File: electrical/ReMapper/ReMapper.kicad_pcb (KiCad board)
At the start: 4 copper layers, 35 x 65 mm, 43 parts, among them J1 ESP_UART0, J2 I2C Display, J3 USB_IN, J4 USB_OUT, J5 Button GND Pad, J9 Button Socket, U1 SPX1117M3-L-3-3/TR, U2 W25Q128JVE, U3 ESP32-S3-WROOM-1-N8R8, U4 RP2040, U5 W25Q128JVE, Y1 12MHZ

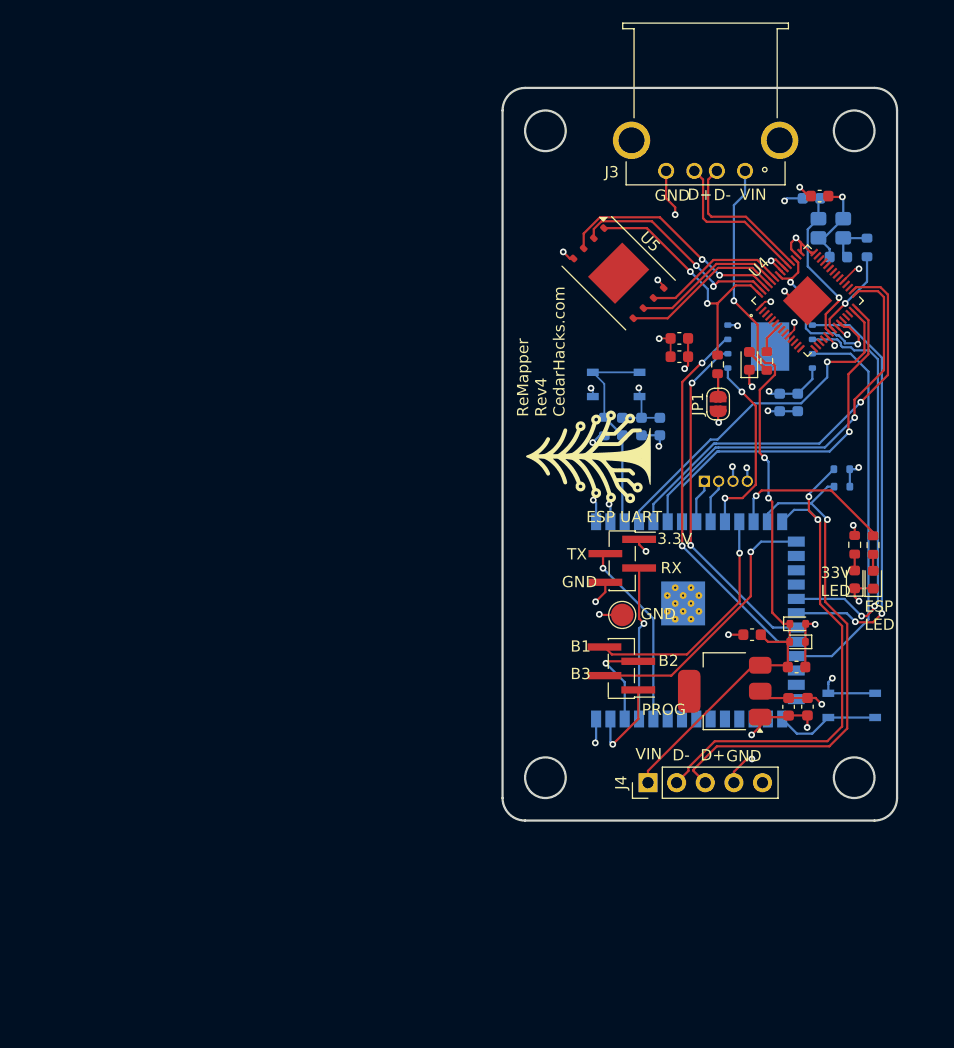
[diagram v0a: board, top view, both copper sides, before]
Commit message: started working on v5
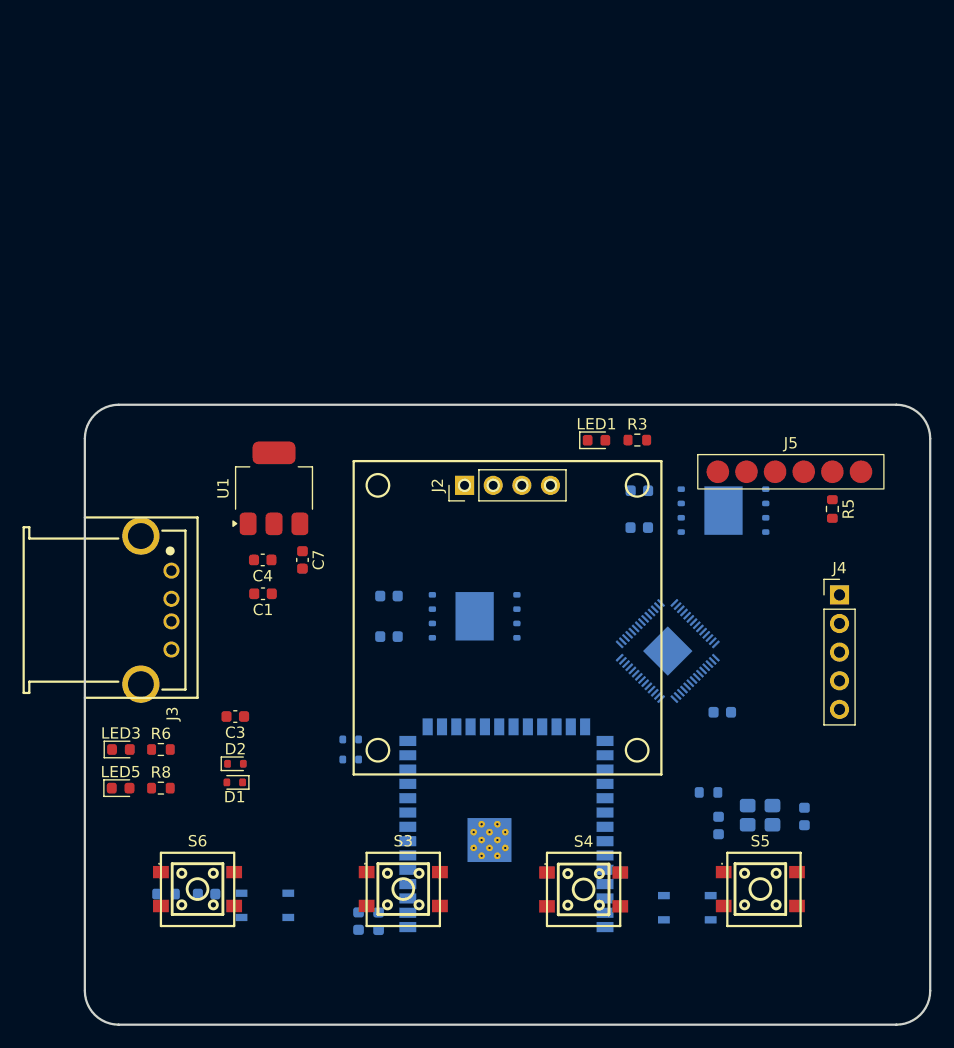
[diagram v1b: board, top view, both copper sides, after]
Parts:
- removed G***: LOGO, LOGO
- removed J1: ESP_UART0, Connector_PinHeader_1.27mm:PinHeader_1x04_P1.27mm_Vertical_SMD_Pin1Right
- removed J9: Button Socket, Connector_PinHeader_1.27mm:PinHeader_1x04_P1.27mm_Vertical_SMD_Pin1Left
- removed JP1: RP2040 Prog, Jumper:SolderJumper-2_P1.3mm_Open_RoundedPad1.0x1.5mm
- added S3: ESP_B1, generated_lscs:SW-SMD_4P-L4.5-W4.5-P3.00-LS6.8, F.Cu at (169.1, 115.0)
- added S4: ESP_B2, generated_lscs:SW-SMD_4P-L4.5-W4.5-P3.00-LS6.8, F.Cu at (185.1, 115.0)
- added S5: ESP_B3, generated_lscs:SW-SMD_4P-L4.5-W4.5-P3.00-LS6.8, F.Cu at (200.8, 115.0)
- added S6: ESP_B4_prog, generated_lscs:SW-SMD_4P-L4.5-W4.5-P3.00-LS6.8, F.Cu at (150.8, 115.0)
- C10, C13, C14, U4, U5: moved to B.Cu
- J2: footprint Connector_PinHeader_1.27mm:PinHeader_1x04_P1.27mm_Vertical -> Connector_PinHeader_2.54mm:PinHeader_1x04_P2.54mm_Vertical; moved to F.Cu
- J5: value Button GND Pad -> Conn_01x06_Pin; footprint TestPoint:TestPoint_Pad_D2.0mm -> cedarhacks:pogo_pin_2.54mm
- moved J3 69.7 mm to (142.6, 90.2), turned to -90 degrees
- moved LED5 69.3 mm to (144.0, 106.0), turned to 0 degrees
- moved R8 66.8 mm to (147.6, 106.0), turned to 180 degrees
- moved LED3 65.6 mm to (144.0, 102.6), turned to 0 degrees
- moved R6 63.9 mm to (147.6, 102.6), turned to 180 degrees
- moved R1 56.9 mm to (148.0, 115.4), turned to 180 degrees
- moved S1 55.7 mm to (156.8, 116.4)
- moved C2 55.5 mm to (151.6, 115.4), turned to 180 degrees
- moved C11 54.8 mm to (204.7, 108.6), turned to 90 degrees
- moved Y1 52.4 mm to (200.7, 108.4), turned to 180 degrees
- moved D1 51.9 mm to (154.1, 105.5), turned to 180 degrees
- moved C12 51.5 mm to (197.0, 109.4), turned to -90 degrees
- moved C8 51.4 mm to (165.1, 117.8), turned to -90 degrees
- moved D2 51.0 mm to (154.2, 103.9), turned to 0 degrees
- moved R2 50.4 mm to (196.2, 106.4), turned to 180 degrees
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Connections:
- J5 pad 1: GND -> /3.3V
- R5 pad 1: Net-(JP1-B) -> /RP2040_PROG
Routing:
- net GND: track 71.6 -> 0.00 mm, vias 26 -> 0
- net /USB_VIN: track 68.6 -> 0.00 mm, vias 3 -> 0
- net /USB_OUT_D-: track 45.8 -> 0.00 mm, vias 2 -> 0
- net /USB_OUT_D+: track 45.8 -> 0.00 mm, vias 1 -> 0
- net /3.3V: track 40.1 -> 0.00 mm, vias 17 -> 0
- net /QSPI_IO0_esp: track 38.3 -> 0.00 mm, vias 2 -> 0
- net /SPI2_MISO: track 37.8 -> 0.00 mm, vias 1 -> 0
- net /QSPI_CLK_esp: track 36.7 -> 0.00 mm, vias 2 -> 0
- net /SPI2_CLK: track 36.4 -> 0.00 mm, vias 1 -> 0
- net /QSPI_IO3_esp: track 35.4 -> 0.00 mm
- net /QSPI_IO2_esp: track 33.8 -> 0.00 mm, vias 2 -> 0
- net /SPI2_CS: track 32.2 -> 0.00 mm, vias 1 -> 0
- net /SPI2_MOSI: track 31.7 -> 0.00 mm, vias 1 -> 0
- net /QSPI_IO1_esp: track 31.1 -> 0.00 mm, vias 2 -> 0
- net /ESP_BUTTON_3: track 24.2 -> 0.00 mm, vias 1 -> 0
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- removed copper zone on In2.Cu, net /3.3V
- removed copper zone on In1.Cu, net GND
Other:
- board size 35 x 65 mm -> 75 x 55 mm
- board text removed: "3.3V"
- board text removed: "33V"
- board text removed: "33V LED"
- board text removed: "B1"
- board text removed: "B2"
- board text removed: "B3"
- board text removed: "CLK"
- board text removed: "D+"
- board text removed: "D-"
- board text removed: "DATA"
- board text removed: "ESP ENB"
- board text removed: "ESP LED"
- board text removed: "ESP UART"
- board text removed: "ESP prog"
- board text removed: "GND"
- board text removed: "PROG"
- board text removed: "RX"
- board text removed: "ReMapper Rev4 CedarHacks.com"
- board text removed: "TX"
- board text removed: "VIN"
